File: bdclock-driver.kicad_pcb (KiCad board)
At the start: 2 copper layers, 34 parts, among them J1 PWR, J2 Ctrl, J3 Kathodes, J4 Anodes A, J5 Anodes B, J6 Anodes C, U1 NE555P, U2 LM7805_TO220, U3 74HC4017, U4 74HC595, U5 74HC595, U6 74HC595, U7 74LS138, U8 74LS138

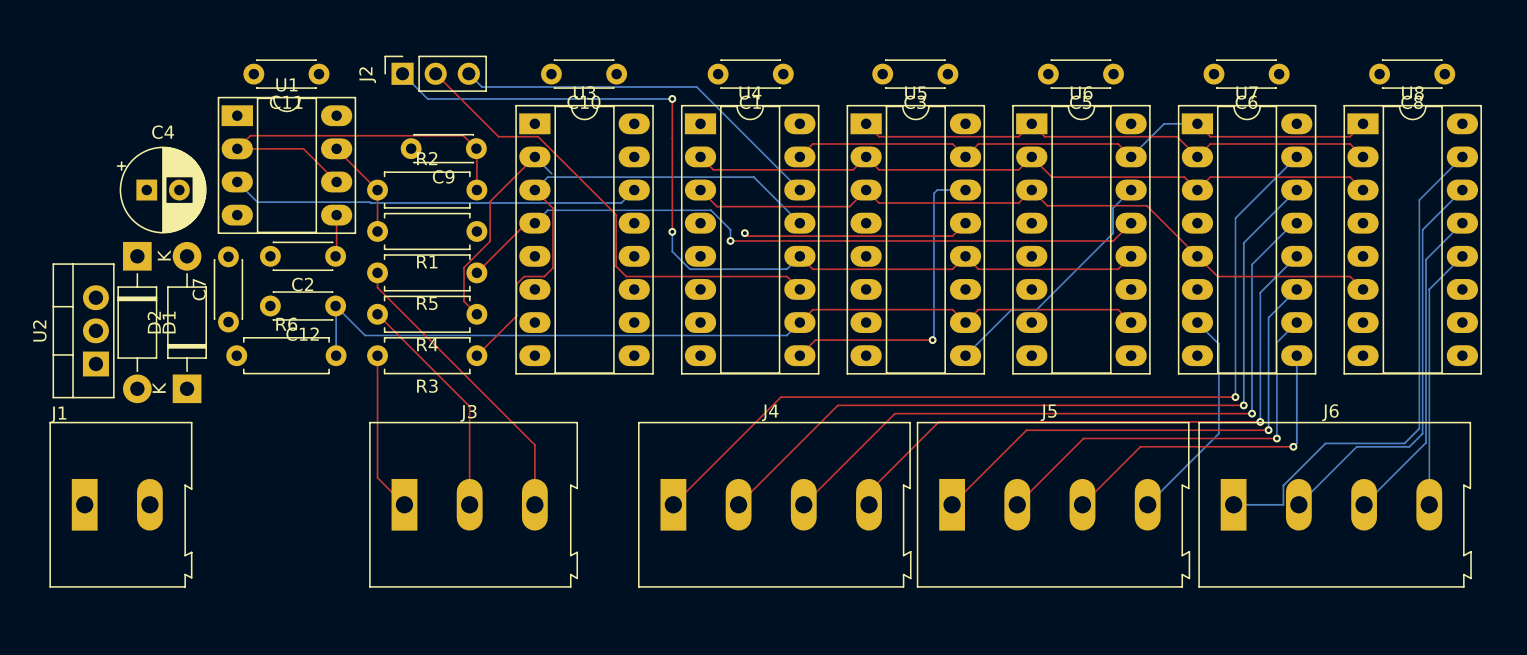
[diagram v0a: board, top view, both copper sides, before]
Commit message: :hammer: Improve PCB layout
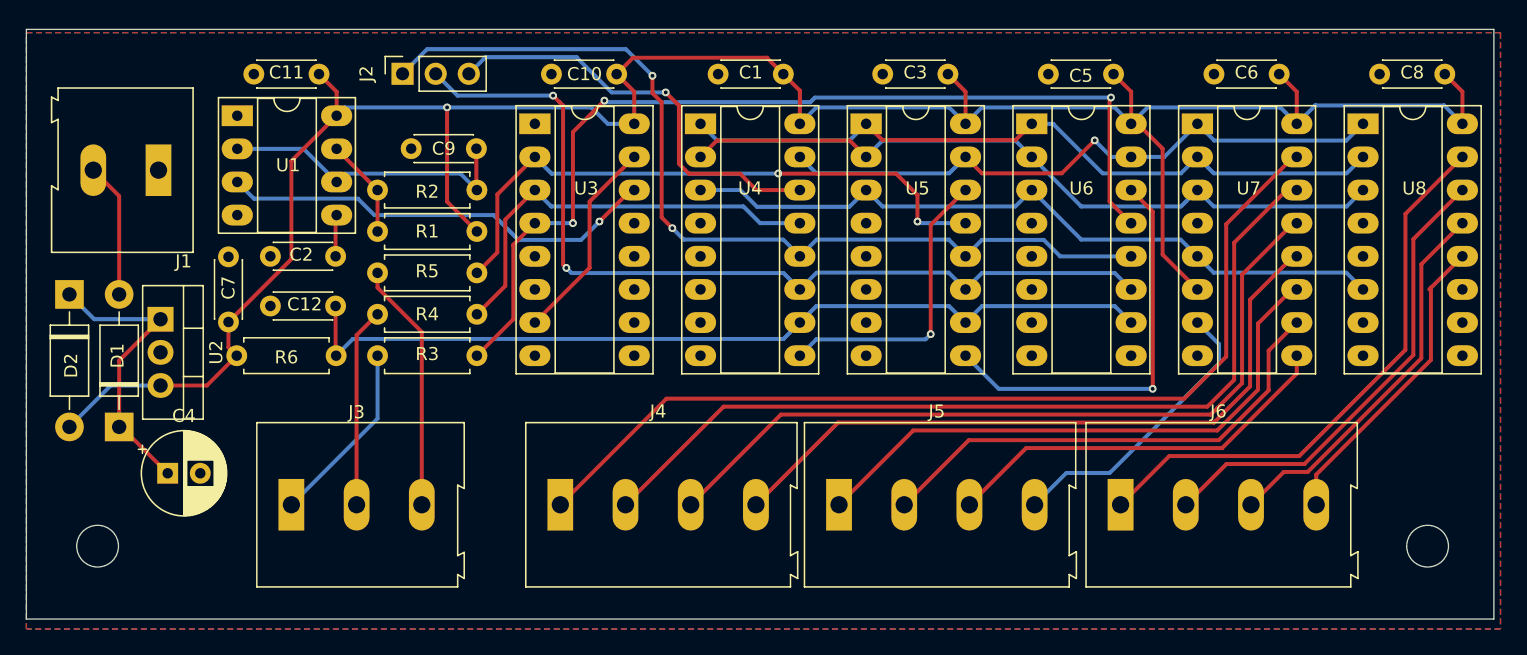
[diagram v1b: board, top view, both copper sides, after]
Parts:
- added REF**: MountingHole_3.2mm_M3, MountingHole:MountingHole_3.2mm_M3, F.Cu at (225.6, 101.6)
- added REF**: MountingHole_3.2mm_M3, MountingHole:MountingHole_3.2mm_M3, F.Cu at (123.6, 101.6)
- moved J1 26.3 mm to (128.2, 72.8), turned to 180 degrees
- moved C4 21.8 mm to (128.9, 96.0)
- moved D1 13.2 mm to (125.2, 92.5), turned to 90 degrees
- moved D2 11.6 mm to (121.4, 82.3), turned to -90 degrees
- moved J5 8.67 mm to (180.4, 98.4)
- moved J6 8.67 mm to (202.0, 98.4)
- moved J3 8.67 mm to (138.4, 98.4)
- moved J4 8.67 mm to (159.1, 98.4)
- moved U2 6.02 mm to (128.4, 84.2), turned to -90 degrees
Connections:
- R3 pad 1: ROW1 -> ROW3
- R4 pad 1: ROW2 -> ROW1
- R5 pad 1: ROW3 -> ROW2
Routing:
- net VCC: track 0.00 -> 185.2 mm, vias 0 -> 1
- net CLK: track 37.1 -> 69.4 mm, vias 0 -> 2
- net Net-(D1-K): track 0.00 -> 22.5 mm
- net ROW3: track 54.2 -> 74.7 mm, vias 1 -> 3
- net Net-(U3-Q3): track 0.00 -> 15.9 mm
- net A2: track 40.8 -> 56.0 mm
- net ROW2: track 34.0 -> 47.1 mm, vias 1 -> 2
- net Net-(U5-QH'): track 19.1 -> 31.3 mm, vias 0 -> 1
- net Net-(D1-A): track 0.00 -> 10.3 mm
- net Net-(U1-THR): track 31.0 -> 23.4 mm
- net Net-(J4-Pin_2): track 60.1 -> 67.6 mm, vias 1 -> 0
- net Net-(J4-Pin_3): track 53.4 -> 60.3 mm, vias 1 -> 0
- net Net-(J4-Pin_1): track 66.9 -> 73.5 mm, vias 1 -> 0
- net Net-(J5-Pin_1): track 38.3 -> 44.9 mm, vias 1 -> 0
- net Net-(J4-Pin_4): track 47.1 -> 53.4 mm, vias 1 -> 0
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- added copper zone on B.Cu, net GND
- added copper zone on F.Cu, net GND
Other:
- board outline added: 112.5 x 45.2 mm

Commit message: :art: Finalize the PCB layout
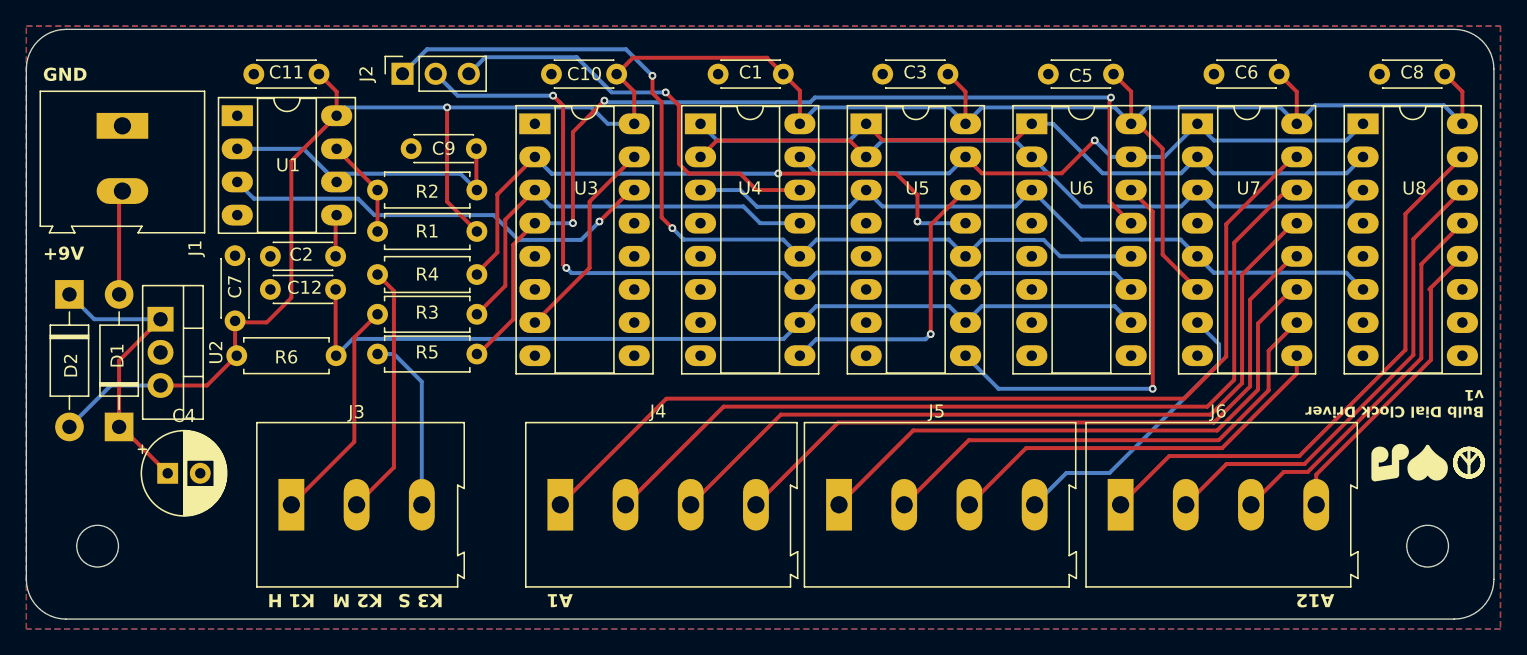
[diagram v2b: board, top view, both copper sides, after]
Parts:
- moved R5 6.22 mm to (152.7, 86.9)
- moved J1 4.38 mm to (125.5, 69.4), turned to -90 degrees
- moved R3 3.18 mm to (152.7, 83.8)
- moved R4 3.05 mm to (152.7, 80.8)
- moved C12 1.27 mm to (141.8, 81.9)
- moved C7 0.51 mm to (134.1, 84.3)
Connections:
- R3 pad 1: ROW3 -> ROW1
- R4 pad 1: ROW1 -> ROW2
- R5 pad 1: ROW2 -> ROW3
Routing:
- net Net-(J3-Pin_3): track 19.2 -> 13.7 mm
- net Net-(J3-Pin_2): track 15.3 -> 19.4 mm
- net Net-(J3-Pin_1): track 14.2 -> 17.3 mm
- net Net-(D1-A): track 10.3 -> 8.03 mm
- net /RST: track 67.9 -> 69.2 mm
- net VCC: track 185.2 -> 186.4 mm
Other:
- outline, holes or cut-outs redrawn
- board text added: "+9V"
- board text added: "A1"
- board text added: "A12"
- board text added: "Bulb Dial Clock Driver"
- board text added: "GND"
- board text added: "K1 H"
- board text added: "K2 M"
- board text added: "K3 S"
- board text added: "https://github.com/penguineer/bdclock-driver"
- board text added: "v1"
